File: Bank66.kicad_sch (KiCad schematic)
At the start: 2 parts, among them U1 XCKU5P-FFVB676

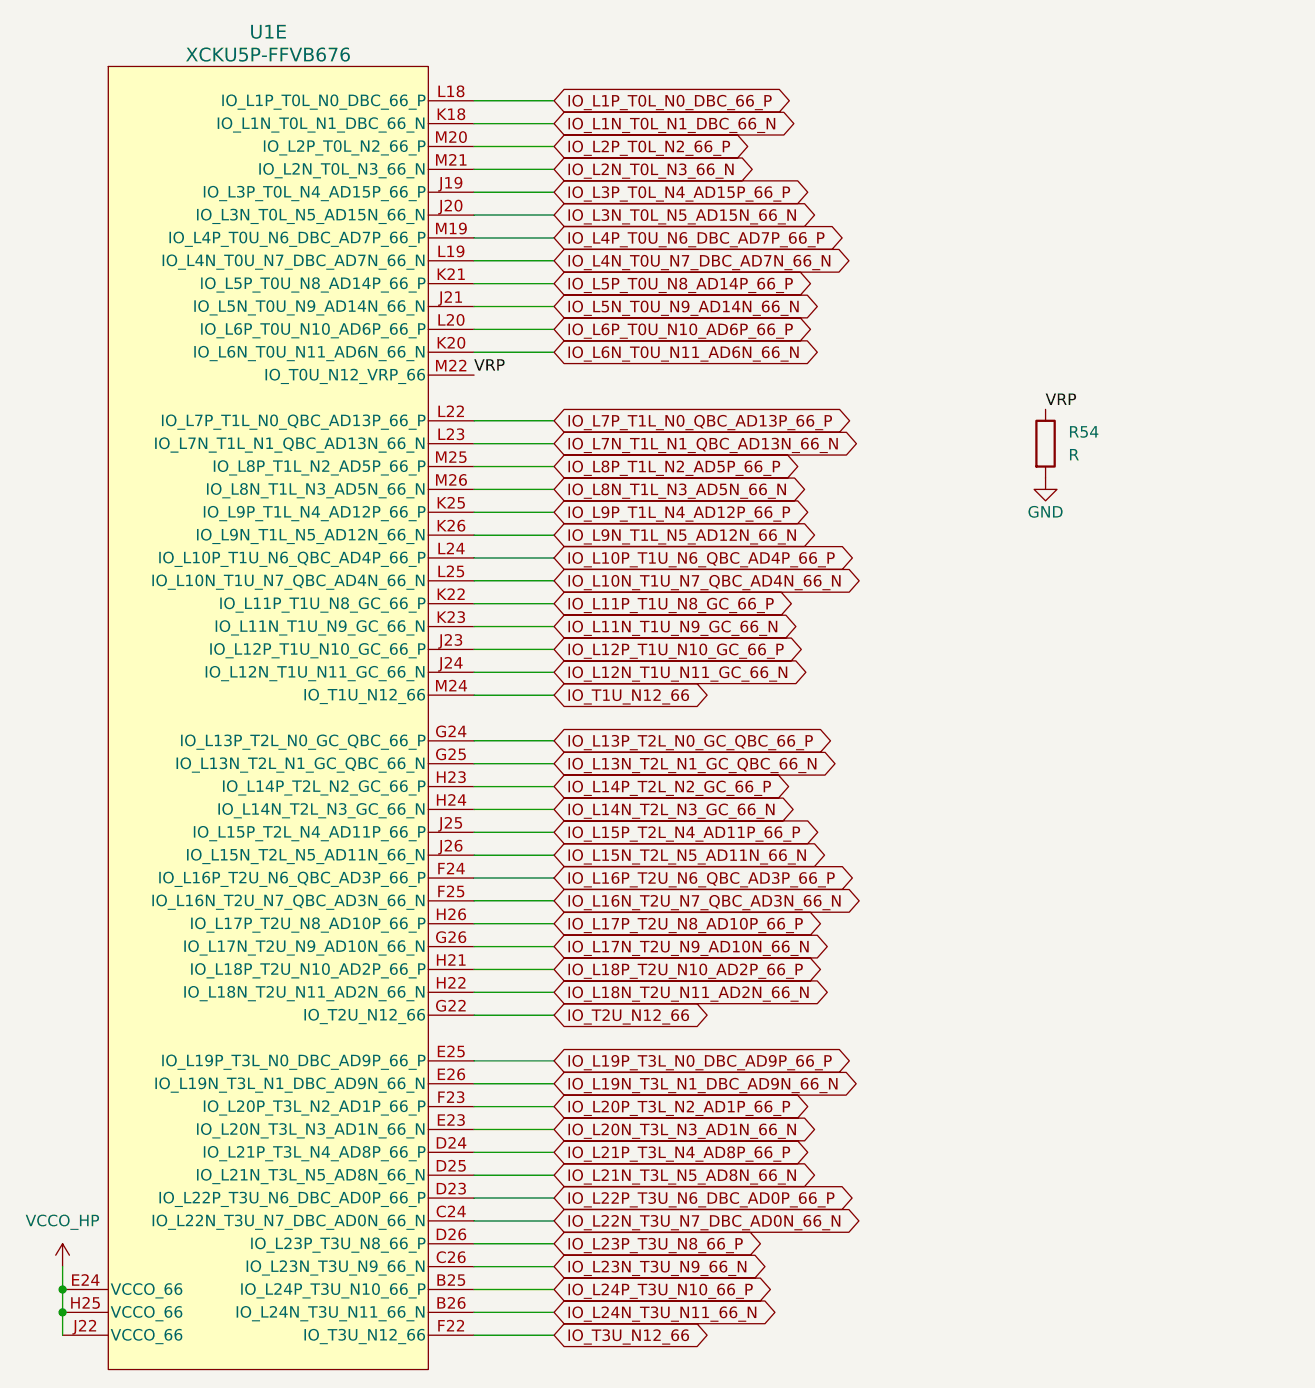
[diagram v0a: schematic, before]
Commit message: pushing the schematics works
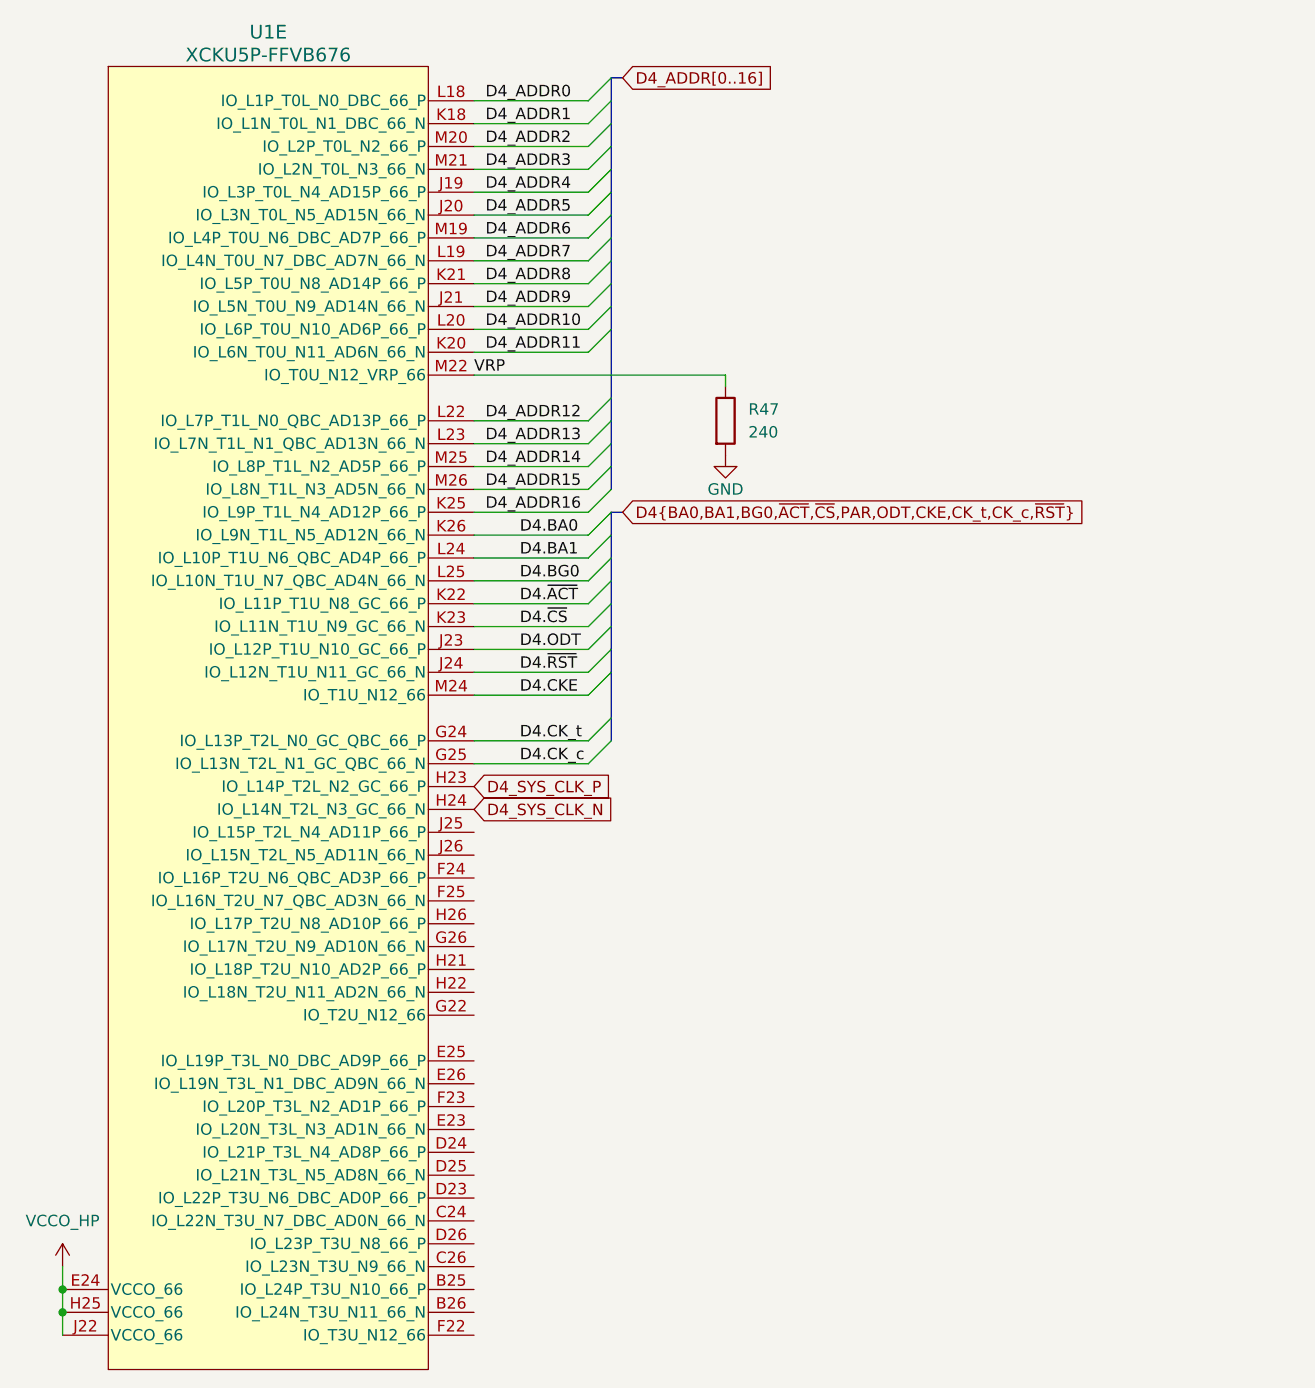
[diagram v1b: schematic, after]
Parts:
- removed R54: R, Resistor_SMD:R_0201_0603Metric, symbol Device:R
- added R47: 240, Resistor_SMD:R_0201_0603Metric, symbol Device:R
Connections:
- net GND: now also R47.2
- net VRP: now also R47.1
- net IO_L10N_T1U_N7_QBC_AD4N_66_N renamed D4.BG0
- net IO_L10P_T1U_N6_QBC_AD4P_66_P renamed D4.BA1
- net IO_L11N_T1U_N9_GC_66_N renamed D4.~{CS}
- net IO_L11P_T1U_N8_GC_66_P renamed D4.~{ACT}
- net IO_L12N_T1U_N11_GC_66_N renamed D4.~{RST}
- net IO_L12P_T1U_N10_GC_66_P renamed D4.ODT
- net IO_L13N_T2L_N1_GC_QBC_66_N renamed D4.CK_c
- net IO_L13P_T2L_N0_GC_QBC_66_P renamed D4.CK_t
- net IO_L14N_T2L_N3_GC_66_N renamed D4_SYS_CLK_N
- net IO_L14P_T2L_N2_GC_66_P renamed D4_SYS_CLK_P
- net IO_L15N_T2L_N5_AD11N_66_N: no longer names the net of U1.J26 (IO_L15N_T2L_N5_AD11N_66_N)
- net IO_L15P_T2L_N4_AD11P_66_P: no longer names the net of U1.J25 (IO_L15P_T2L_N4_AD11P_66_P)
- net IO_L16N_T2U_N7_QBC_AD3N_66_N: no longer names the net of U1.F25 (IO_L16N_T2U_N7_QBC_AD3N_66_N)
- net IO_L16P_T2U_N6_QBC_AD3P_66_P: no longer names the net of U1.F24 (IO_L16P_T2U_N6_QBC_AD3P_66_P)
- net IO_L17N_T2U_N9_AD10N_66_N: no longer names the net of U1.G26 (IO_L17N_T2U_N9_AD10N_66_N)
- net IO_L17P_T2U_N8_AD10P_66_P: no longer names the net of U1.H26 (IO_L17P_T2U_N8_AD10P_66_P)
- net IO_L18N_T2U_N11_AD2N_66_N: no longer names the net of U1.H22 (IO_L18N_T2U_N11_AD2N_66_N)
- net IO_L18P_T2U_N10_AD2P_66_P: no longer names the net of U1.H21 (IO_L18P_T2U_N10_AD2P_66_P)
- net IO_L19N_T3L_N1_DBC_AD9N_66_N: no longer names the net of U1.E26 (IO_L19N_T3L_N1_DBC_AD9N_66_N)
- net IO_L19P_T3L_N0_DBC_AD9P_66_P: no longer names the net of U1.E25 (IO_L19P_T3L_N0_DBC_AD9P_66_P)
- net IO_L1N_T0L_N1_DBC_66_N renamed D4_ADDR1
- net IO_L1P_T0L_N0_DBC_66_P renamed D4_ADDR0
- net IO_L20N_T3L_N3_AD1N_66_N: no longer names the net of U1.E23 (IO_L20N_T3L_N3_AD1N_66_N)
- net IO_L20P_T3L_N2_AD1P_66_P: no longer names the net of U1.F23 (IO_L20P_T3L_N2_AD1P_66_P)
- net IO_L21N_T3L_N5_AD8N_66_N: no longer names the net of U1.D25 (IO_L21N_T3L_N5_AD8N_66_N)
- net IO_L21P_T3L_N4_AD8P_66_P: no longer names the net of U1.D24 (IO_L21P_T3L_N4_AD8P_66_P)
- net IO_L22N_T3U_N7_DBC_AD0N_66_N: no longer names the net of U1.C24 (IO_L22N_T3U_N7_DBC_AD0N_66_N)
- net IO_L22P_T3U_N6_DBC_AD0P_66_P: no longer names the net of U1.D23 (IO_L22P_T3U_N6_DBC_AD0P_66_P)
- net IO_L23N_T3U_N9_66_N: no longer names the net of U1.C26 (IO_L23N_T3U_N9_66_N)
- net IO_L23P_T3U_N8_66_P: no longer names the net of U1.D26 (IO_L23P_T3U_N8_66_P)
- net IO_L24N_T3U_N11_66_N: no longer names the net of U1.B26 (IO_L24N_T3U_N11_66_N)
- net IO_L24P_T3U_N10_66_P: no longer names the net of U1.B25 (IO_L24P_T3U_N10_66_P)
- net IO_L2N_T0L_N3_66_N renamed D4_ADDR3
- net IO_L2P_T0L_N2_66_P renamed D4_ADDR2
- net IO_L3N_T0L_N5_AD15N_66_N renamed D4_ADDR5
- net IO_L3P_T0L_N4_AD15P_66_P renamed D4_ADDR4
- net IO_L4N_T0U_N7_DBC_AD7N_66_N renamed D4_ADDR7
- net IO_L4P_T0U_N6_DBC_AD7P_66_P renamed D4_ADDR6
- net IO_L5N_T0U_N9_AD14N_66_N renamed D4_ADDR9
- net IO_L5P_T0U_N8_AD14P_66_P renamed D4_ADDR8
- net IO_L6N_T0U_N11_AD6N_66_N renamed D4_ADDR11
- net IO_L6P_T0U_N10_AD6P_66_P renamed D4_ADDR10
- net IO_L7N_T1L_N1_QBC_AD13N_66_N renamed D4_ADDR13
- net IO_L7P_T1L_N0_QBC_AD13P_66_P renamed D4_ADDR12
- net IO_L8N_T1L_N3_AD5N_66_N renamed D4_ADDR15
- net IO_L8P_T1L_N2_AD5P_66_P renamed D4_ADDR14
- net IO_L9N_T1L_N5_AD12N_66_N renamed D4.BA0
- net IO_L9P_T1L_N4_AD12P_66_P renamed D4_ADDR16
- net IO_T1U_N12_66 renamed D4.CKE
- net IO_T2U_N12_66: no longer names the net of U1.G22 (IO_T2U_N12_66)
- net IO_T3U_N12_66: no longer names the net of U1.F22 (IO_T3U_N12_66)
